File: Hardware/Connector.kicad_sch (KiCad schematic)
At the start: 6 parts, among them J1 Conn_02x16_Counter_Clockwise, J2 FTSH-107-01-L-D-K

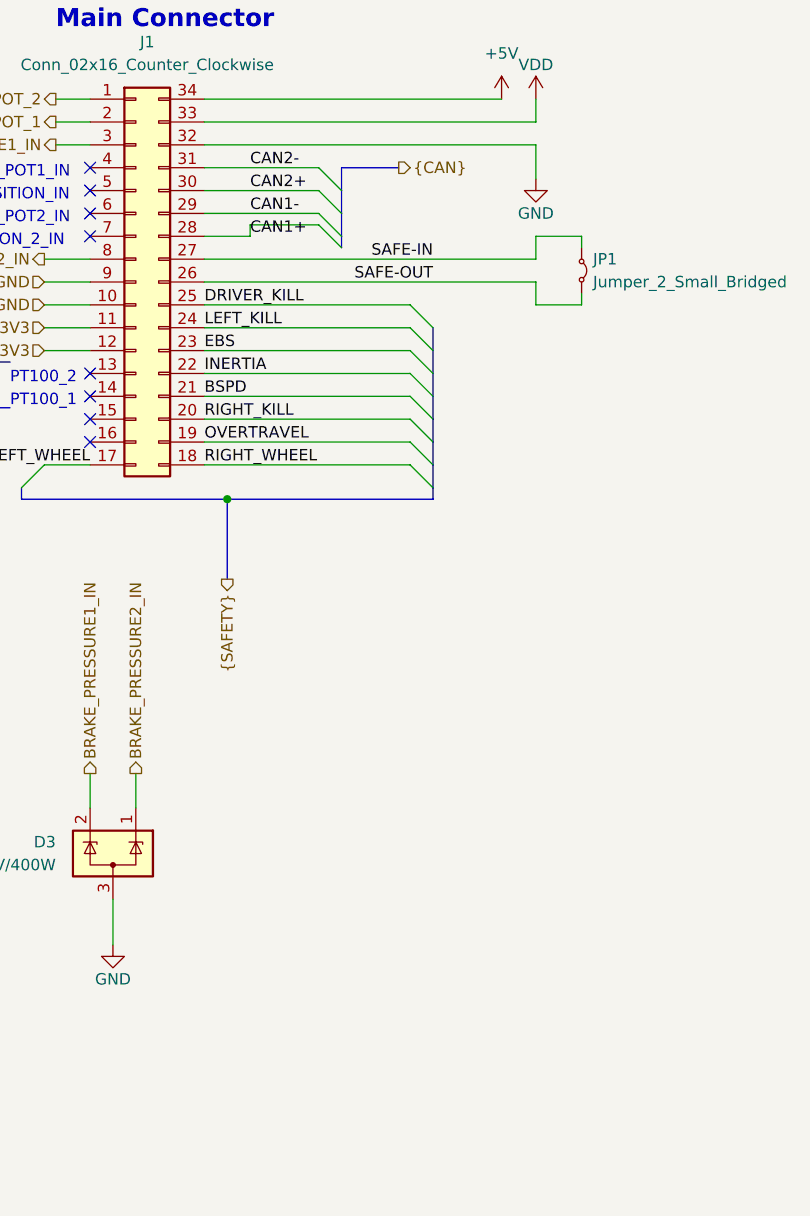
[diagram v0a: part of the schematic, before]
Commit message: Changes in CAN section
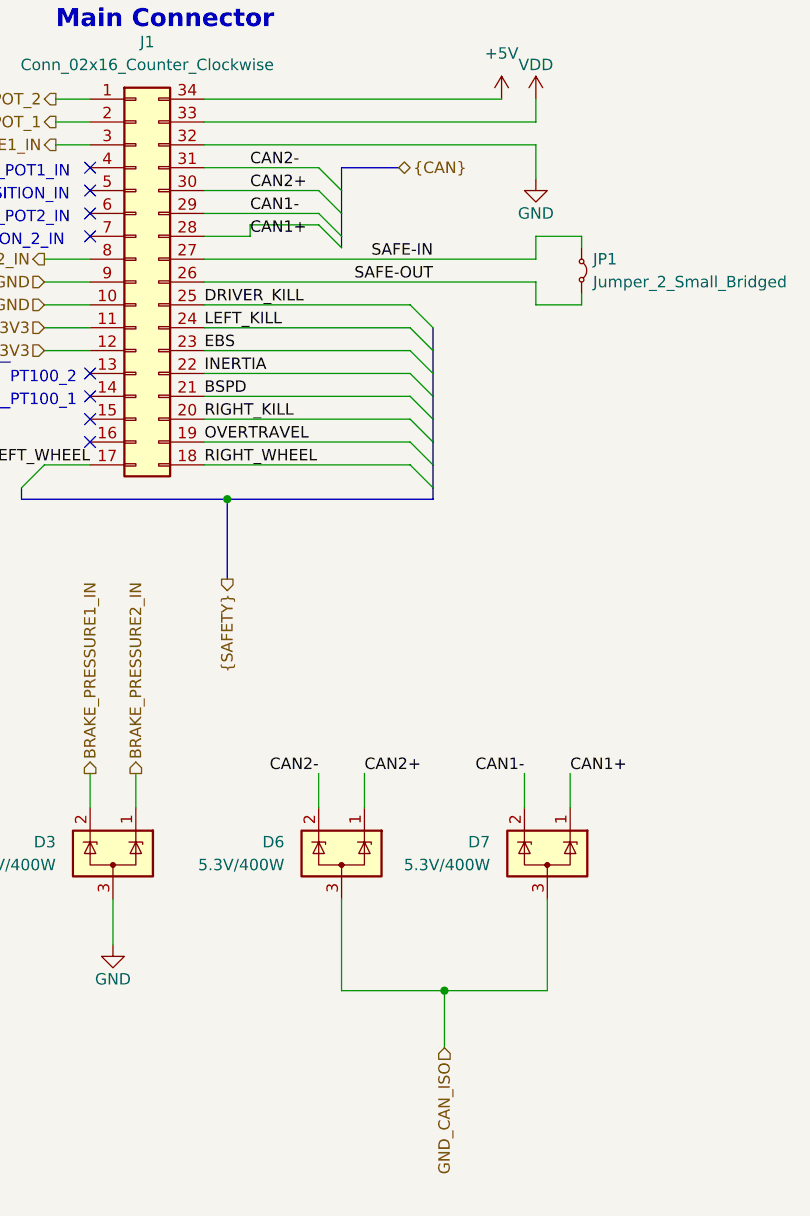
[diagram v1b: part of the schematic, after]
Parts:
- added D6, D7: 5.3V/400W, Package_TO_SOT_SMD:SOT-23-3, symbol Power_Protection:ESDA5V3L
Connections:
- net CAN1+: now also D7.1 (K)
- net CAN1-: now also D7.2 (K)
- net CAN2+: now also D6.1 (K)
- net CAN2-: now also D6.2 (K)
- new net GND_CAN_ISO: D6.3 (A), D7.3 (A)
